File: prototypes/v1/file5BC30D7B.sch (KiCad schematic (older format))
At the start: 4 parts, among them J1 Conn_01x08_Male, U16 68681, U17 MAX233-SO, U18 MAX233-SO

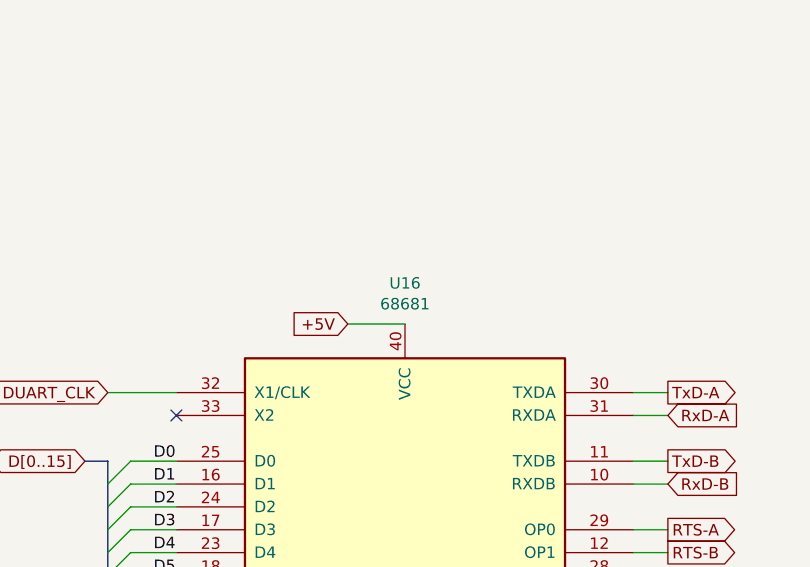
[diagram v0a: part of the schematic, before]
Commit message: finish logic
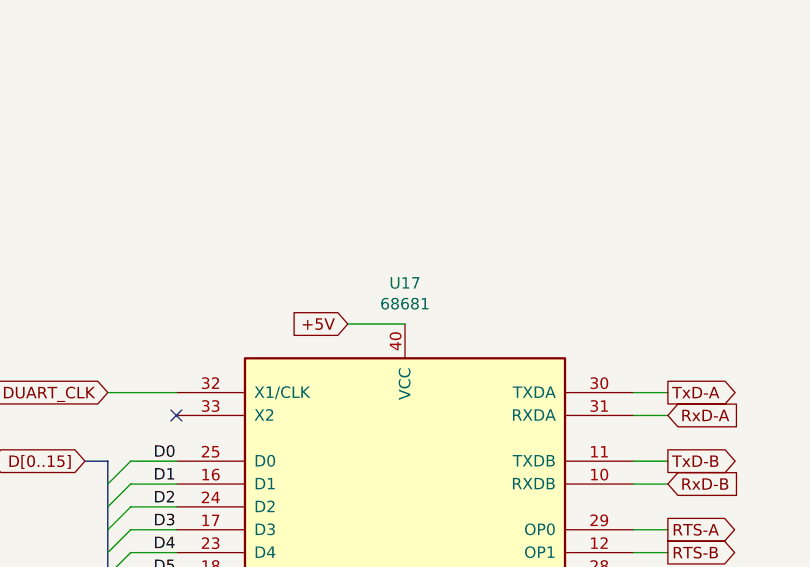
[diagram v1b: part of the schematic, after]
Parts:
- renumbered U16 to U17, U17 to U18, U18 to U19
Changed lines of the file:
@@
 P 2400 3850
 AR Path="/5BC313C4" Ref="U?"  Part="1"
-AR Path="/5BC30D7C/5BC313C4" Ref="U16"  Part="1"
-F 0 "U16" H 2400 5528 50  0000 C CNN
+AR Path="/5BC30D7C/5BC313C4" Ref="U17"  Part="1"
+F 0 "U17" H 2400 5528 50  0000 C CNN
 F 1 "68681" H 2400 5437 50  0000 C CNN
 F 2 "" H 2400 3850 50  0001 C CNN
@@
 P 2600 5250
 AR Path="/5BC313CC" Ref="#PWR?"  Part="1"
-AR Path="/5BC30D7C/5BC313CC" Ref="#PWR0120"  Part="1"
-F 0 "#PWR0120" H 2600 5000 50  0001 C CNN
+AR Path="/5BC30D7C/5BC313CC" Ref="#PWR015"  Part="1"
+F 0 "#PWR015" H 2600 5000 50  0001 C CNN
 F 1 "GND" H 2605 5077 50  0000 C CNN
 F 2 "" H 2600 5250 50  0001 C CNN
@@
 P 5700 2050
 AR Path="/5BC393D4" Ref="U?"  Part="1"
-AR Path="/5BC30D7C/5BC393D4" Ref="U17"  Part="1"
-F 0 "U17" H 5700 3428 50  0000 C CNN
+AR Path="/5BC30D7C/5BC393D4" Ref="U18"  Part="1"
+F 0 "U18" H 5700 3428 50  0000 C CNN
 F 1 "MAX233-SO" H 5700 3337 50  0000 C CNN
 F 2 "" H 5750 1000 50  0001 L CNN
@@
 P 5700 3350
 AR Path="/5BC393DB" Ref="#PWR?"  Part="1"
-AR Path="/5BC30D7C/5BC393DB" Ref="#PWR0121"  Part="1"
-F 0 "#PWR0121" H 5700 3100 50  0001 C CNN
+AR Path="/5BC30D7C/5BC393DB" Ref="#PWR016"  Part="1"
+F 0 "#PWR016" H 5700 3100 50  0001 C CNN
 F 1 "GND" H 5705 3177 50  0000 C CNN
 F 2 "" H 5700 3350 50  0001 C CNN
@@
 P 5750 5150
 AR Path="/5BC3998B" Ref="U?"  Part="1"
-AR Path="/5BC30D7C/5BC3998B" Ref="U18"  Part="1"
-F 0 "U18" H 5750 6528 50  0000 C CNN
+AR Path="/5BC30D7C/5BC3998B" Ref="U19"  Part="1"
+F 0 "U19" H 5750 6528 50  0000 C CNN
 F 1 "MAX233-SO" H 5750 6437 50  0000 C CNN
 F 2 "" H 5800 4100 50  0001 L CNN
@@
 P 5750 6450
 AR Path="/5BC39992" Ref="#PWR?"  Part="1"
-AR Path="/5BC30D7C/5BC39992" Ref="#PWR0122"  Part="1"
-F 0 "#PWR0122" H 5750 6200 50  0001 C CNN
+AR Path="/5BC30D7C/5BC39992" Ref="#PWR017"  Part="1"
+F 0 "#PWR017" H 5750 6200 50  0001 C CNN
 F 1 "GND" H 5755 6277 50  0000 C CNN
 F 2 "" H 5750 6450 50  0001 C CNN

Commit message: optimized logic
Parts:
- removed U18, U19: MAX233-SO, symbol raven-prototypes:MAX233-SO
- added J2: Ext_Signal, symbol Connector:Conn_01x14_Male
- added U17, U18: MAX233-DIP, symbol raven-prototypes:MAX233-DIP
- J1: value Conn_01x08_Male -> Serial_Connections
- U16: renamed from U17; footprint (none) -> Package_DIP:DIP-40_W15.24mm
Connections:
- net labels added: A16, A17, A18, A19, A20, A21, A22, A23, EXT_DUART_CS, EXT_RAM_CS, EXT_ROM_CS, LDS, UDS
- wire segments 81 -> 91
- no-connect marks 17 -> 18
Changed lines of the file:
@@
 EELAYER 26 0
 EELAYER END
-$Descr A4 11693 8268
+$Descr USLegal 14000 8500
 encoding utf-8
 Sheet 3 4
@@
 P 2400 3850
 AR Path="/5BC313C4" Ref="U?"  Part="1"
-AR Path="/5BC30D7C/5BC313C4" Ref="U17"  Part="1"
-F 0 "U17" H 2400 5528 50  0000 C CNN
+AR Path="/5BC30D7C/5BC313C4" Ref="U16"  Part="1"
+F 0 "U16" H 2400 5528 50  0000 C CNN
 F 1 "68681" H 2400 5437 50  0000 C CNN
-F 2 "" H 2400 3850 50  0001 C CNN
+F 2 "Package_DIP:DIP-40_W15.24mm" H 2400 3850 50  0001 C CNN
 F 3 "" H 2400 3850 50  0001 C CNN
 	1    2400 3850
@@
 	1400 4350 1100 4350
 $Comp
-L raven-prototypes:MAX233-SO U?
-U 1 1 5BC393D4
-P 5700 2050
-AR Path="/5BC393D4" Ref="U?"  Part="1"
-AR Path="/5BC30D7C/5BC393D4" Ref="U18"  Part="1"
-F 0 "U18" H 5700 3428 50  0000 C CNN
-F 1 "MAX233-SO" H 5700 3337 50  0000 C CNN
-F 2 "" H 5750 1000 50  0001 L CNN
-F 3 "" H 5700 2150 50  0001 C CNN
-	1    5700 2050
-	1    0    0    -1
-$EndComp
-$Comp
 L power:GND #PWR?
 U 1 1 5BC393DB
-P 5700 3350
+P 5800 3350
 AR Path="/5BC393DB" Ref="#PWR?"  Part="1"
-AR Path="/5BC30D7C/5BC393DB" Ref="#PWR016"  Part="1"
-F 0 "#PWR016" H 5700 3100 50  0001 C CNN
-F 1 "GND" H 5705 3177 50  0000 C CNN
-F 2 "" H 5700 3350 50  0001 C CNN
-F 3 "" H 5700 3350 50  0001 C CNN
-	1    5700 3350
+AR Path="/5BC30D7C/5BC393DB" Ref="#PWR018"  Part="1"
+F 0 "#PWR018" H 5800 3100 50  0001 C CNN
+F 1 "GND" H 5805 3177 50  0000 C CNN
+F 2 "" H 5800 3350 50  0001 C CNN
+F 3 "" H 5800 3350 50  0001 C CNN
+	1    5800 3350
 	1    0    0    -1
 $EndComp
@@
 	5800 3250 5800 3350
 Wire Wire Line
-	5800 3350 5700 3350
-Wire Wire Line
 	5600 3250 5600 3350
-Wire Wire Line
-	5600 3350 5700 3350
-Connection ~ 5700 3350
 Text GLabel 5450 850  0    50   Input ~ 0
 +5V
@@
 	5450 850  5700 850
 $Comp
-L raven-prototypes:MAX233-SO U?
-U 1 1 5BC3998B
-P 5750 5150
-AR Path="/5BC3998B" Ref="U?"  Part="1"
-AR Path="/5BC30D7C/5BC3998B" Ref="U19"  Part="1"
-F 0 "U19" H 5750 6528 50  0000 C CNN
-F 1 "MAX233-SO" H 5750 6437 50  0000 C CNN
-F 2 "" H 5800 4100 50  0001 L CNN
-F 3 "" H 5750 5250 50  0001 C CNN
-	1    5750 5150
-	1    0    0    -1
-$EndComp
-$Comp
 L power:GND #PWR?
 U 1 1 5BC39992
-P 5750 6450
+P 5850 6450
 AR Path="/5BC39992" Ref="#PWR?"  Part="1"
-AR Path="/5BC30D7C/5BC39992" Ref="#PWR017"  Part="1"
-F 0 "#PWR017" H 5750 6200 50  0001 C CNN
-F 1 "GND" H 5755 6277 50  0000 C CNN
-F 2 "" H 5750 6450 50  0001 C CNN
-F 3 "" H 5750 6450 50  0001 C CNN
-	1    5750 6450
+AR Path="/5BC30D7C/5BC39992" Ref="#PWR019"  Part="1"
+F 0 "#PWR019" H 5850 6200 50  0001 C CNN
+F 1 "GND" H 5855 6277 50  0000 C CNN
+F 2 "" H 5850 6450 50  0001 C CNN
+F 3 "" H 5850 6450 50  0001 C CNN
+	1    5850 6450
 	1    0    0    -1
 $EndComp
@@
 	5850 6350 5850 6450
 Wire Wire Line
-	5850 6450 5750 6450
-Wire Wire Line
 	5650 6350 5650 6450
-Wire Wire Line
-	5650 6450 5750 6450
-Connection ~ 5750 6450
 Text GLabel 5500 3950 0    50   Input ~ 0
 +5V
@@
 P 9400 3650
 F 0 "J1" H 9373 3623 50  0000 R CNN
-F 1 "Conn_01x08_Male" H 9373 3532 50  0000 R CNN
+F 1 "Serial_Connections" H 9373 3532 50  0000 R CNN
 F 2 "" H 9400 3650 50  0001 C CNN
 F 3 "~" H 9400 3650 50  0001 C CNN
@@
 Wire Wire Line
 	8950 4050 9200 4050
+$Comp
+L Connector:Conn_01x14_Male J2
+U 1 1 5BCD7D12
+P 11150 3450
+F 0 "J2" H 11256 4228 50  0000 C CNN
+F 1 "Ext_Signal" H 11256 4137 50  0000 C CNN
+F 2 "" H 11150 3450 50  0001 C CNN
+F 3 "~" H 11150 3450 50  0001 C CNN
+	1    11150 3450
+	1    0    0    -1
+$EndComp
+Wire Wire Line
+	11350 2850 11550 2850
+Wire Wire Line
+	11350 2950 11550 2950
+Wire Wire Line
+	11350 3050 11550 3050
+Wire Wire Line
+	11350 3150 11550 3150
+Wire Wire Line
+	11350 3250 11550 3250
+Wire Wire Line
+	11350 3350 11550 3350
+Wire Wire Line
+	11350 3450 11550 3450
+Wire Wire Line
+	11350 3550 11550 3550
+Wire Wire Line
+	11350 3650 11550 3650
+Wire Wire Line
+	11350 3750 11550 3750
+Wire Wire Line
+	11350 3850 11550 3850
+Wire Wire Line
+	11350 3950 11550 3950
+Wire Wire Line
+	11350 4050 11550 4050
+Wire Wire Line
+	11350 4150 11550 4150
+Text GLabel 11550 2850 2    50   Output ~ 0
+EXT_ROM_CS
+Text GLabel 11550 2950 2    50   Output ~ 0
+EXT_RAM_CS
+Text GLabel 11550 3050 2    50   Output ~ 0
+EXT_DUART_CS
+Text GLabel 11550 3150 2    50   Input ~ 0
+UDS
+Text GLabel 11550 3250 2    50   Input ~ 0
+LDS
+Entry Wire Line
+	11550 4150 11650 4250
+Entry Wire Line
+	11550 4050 11650 4150
+Entry Wire Line
+	11550 3950 11650 4050
+Entry Wire Line
+	11550 3850 11650 3950
+Entry Wire Line
+	11550 3750 11650 3850
+Entry Wire Line
+	11550 3650 11650 3750
+Entry Wire Line
+	11550 3550 11650 3650
+Entry Wire Line
+	11550 3450 11650 3550
+Wire Bus Line
+	11650 3500 11750 3500
+Text GLabel 11750 3500 2    50   Input ~ 0
+A[1..23]
+Text Label 11400 3450 0    50   ~ 0
+A16
+Text Label 11400 3550 0    50   ~ 0
+A17
+Text Label 11400 3650 0    50   ~ 0
+A18
+Text Label 11400 3750 0    50   ~ 0
+A19
+Text Label 11400 3850 0    50   ~ 0
+A20
+Text Label 11400 3950 0    50   ~ 0
+A21
+Text Label 11400 4050 0    50   ~ 0
+A22
+Text Label 11400 4150 0    50   ~ 0
+A23
+NoConn ~ 11550 3350
+$Comp
+L raven-prototypes:MAX233-DIP U18
+U 1 1 5BD453EC
+P 5750 5150
+F 0 "U18" H 5750 6528 50  0000 C CNN
+F 1 "MAX233-DIP" H 5750 6437 50  0000 C CNN
+F 2 "" H 5800 4100 50  0001 L CNN
+F 3 "" H 5750 5250 50  0001 C CNN
+	1    5750 5150
+	1    0    0    -1
+$EndComp
+$Comp
+L raven-prototypes:MAX233-DIP U17
+U 1 1 5BD45448
+P 5700 2050
+F 0 "U17" H 5700 3428 50  0000 C CNN
+F 1 "MAX233-DIP" H 5700 3337 50  0000 C CNN
+F 2 "" H 5750 1000 50  0001 L CNN
+F 3 "" H 5700 2150 50  0001 C CNN
+	1    5700 2050
+	1    0    0    -1
+$EndComp
+$Comp
+L power:GND #PWR?
+U 1 1 5BD6853B
+P 5600 3350
+AR Path="/5BD6853B" Ref="#PWR?"  Part="1"
+AR Path="/5BC30D7C/5BD6853B" Ref="#PWR016"  Part="1"
+F 0 "#PWR016" H 5600 3100 50  0001 C CNN
+F 1 "GND" H 5605 3177 50  0000 C CNN
+F 2 "" H 5600 3350 50  0001 C CNN
+F 3 "" H 5600 3350 50  0001 C CNN
+	1    5600 3350
+	1    0    0    -1
+$EndComp
+$Comp
+L power:GND #PWR?
+U 1 1 5BD685AC
+P 5650 6450
+AR Path="/5BD685AC" Ref="#PWR?"  Part="1"
+AR Path="/5BC30D7C/5BD685AC" Ref="#PWR017"  Part="1"
+F 0 "#PWR017" H 5650 6200 50  0001 C CNN
+F 1 "GND" H 5655 6277 50  0000 C CNN
+F 2 "" H 5650 6450 50  0001 C CNN
+F 3 "" H 5650 6450 50  0001 C CNN
+	1    5650 6450
+	1    0    0    -1
+$EndComp
 Wire Bus Line
 	1100 3850 1100 4250
 Wire Bus Line
 	1100 2950 1100 3750
+Wire Bus Line
+	11650 3500 11650 4250
 $EndSCHEMATC

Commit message: gerbers created, Rev 0 sent to manufacturer
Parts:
- J1: footprint (none) -> Pin_Headers:Pin_Header_Straight_1x08_Pitch2.54mm
- J2: footprint (none) -> Pin_Headers:Pin_Header_Straight_1x14_Pitch2.54mm
- U17, U18: footprint (none) -> Package_DIP:DIP-20_W7.62mm
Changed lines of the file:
@@
 F 0 "J1" H 9373 3623 50  0000 R CNN
 F 1 "Serial_Connections" H 9373 3532 50  0000 R CNN
-F 2 "" H 9400 3650 50  0001 C CNN
+F 2 "Pin_Headers:Pin_Header_Straight_1x08_Pitch2.54mm" H 9400 3650 50  0001 C CNN
 F 3 "~" H 9400 3650 50  0001 C CNN
 	1    9400 3650
@@
 F 0 "J2" H 11256 4228 50  0000 C CNN
 F 1 "Ext_Signal" H 11256 4137 50  0000 C CNN
-F 2 "" H 11150 3450 50  0001 C CNN
+F 2 "Pin_Headers:Pin_Header_Straight_1x14_Pitch2.54mm" H 11150 3450 50  0001 C CNN
 F 3 "~" H 11150 3450 50  0001 C CNN
 	1    11150 3450
@@
 F 0 "U18" H 5750 6528 50  0000 C CNN
 F 1 "MAX233-DIP" H 5750 6437 50  0000 C CNN
-F 2 "" H 5800 4100 50  0001 L CNN
+F 2 "Package_DIP:DIP-20_W7.62mm" H 5800 4100 50  0001 L CNN
 F 3 "" H 5750 5250 50  0001 C CNN
 	1    5750 5150
@@
 F 0 "U17" H 5700 3428 50  0000 C CNN
 F 1 "MAX233-DIP" H 5700 3337 50  0000 C CNN
-F 2 "" H 5750 1000 50  0001 L CNN
+F 2 "Package_DIP:DIP-20_W7.62mm" H 5750 1000 50  0001 L CNN
 F 3 "" H 5700 2150 50  0001 C CNN
 	1    5700 2050
